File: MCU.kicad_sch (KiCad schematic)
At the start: 31 parts, among them J15 Display, J18 MEM2061-01-188-00-A_REVA, J19 TYPE-C 15PIN, Q1 PMBT6428,215, Q2 PMBT6428,215, SW5 Reset, SW6 Boot, U5 ESP32-WROOM-32E 4MB, U6 CP2102-GMR

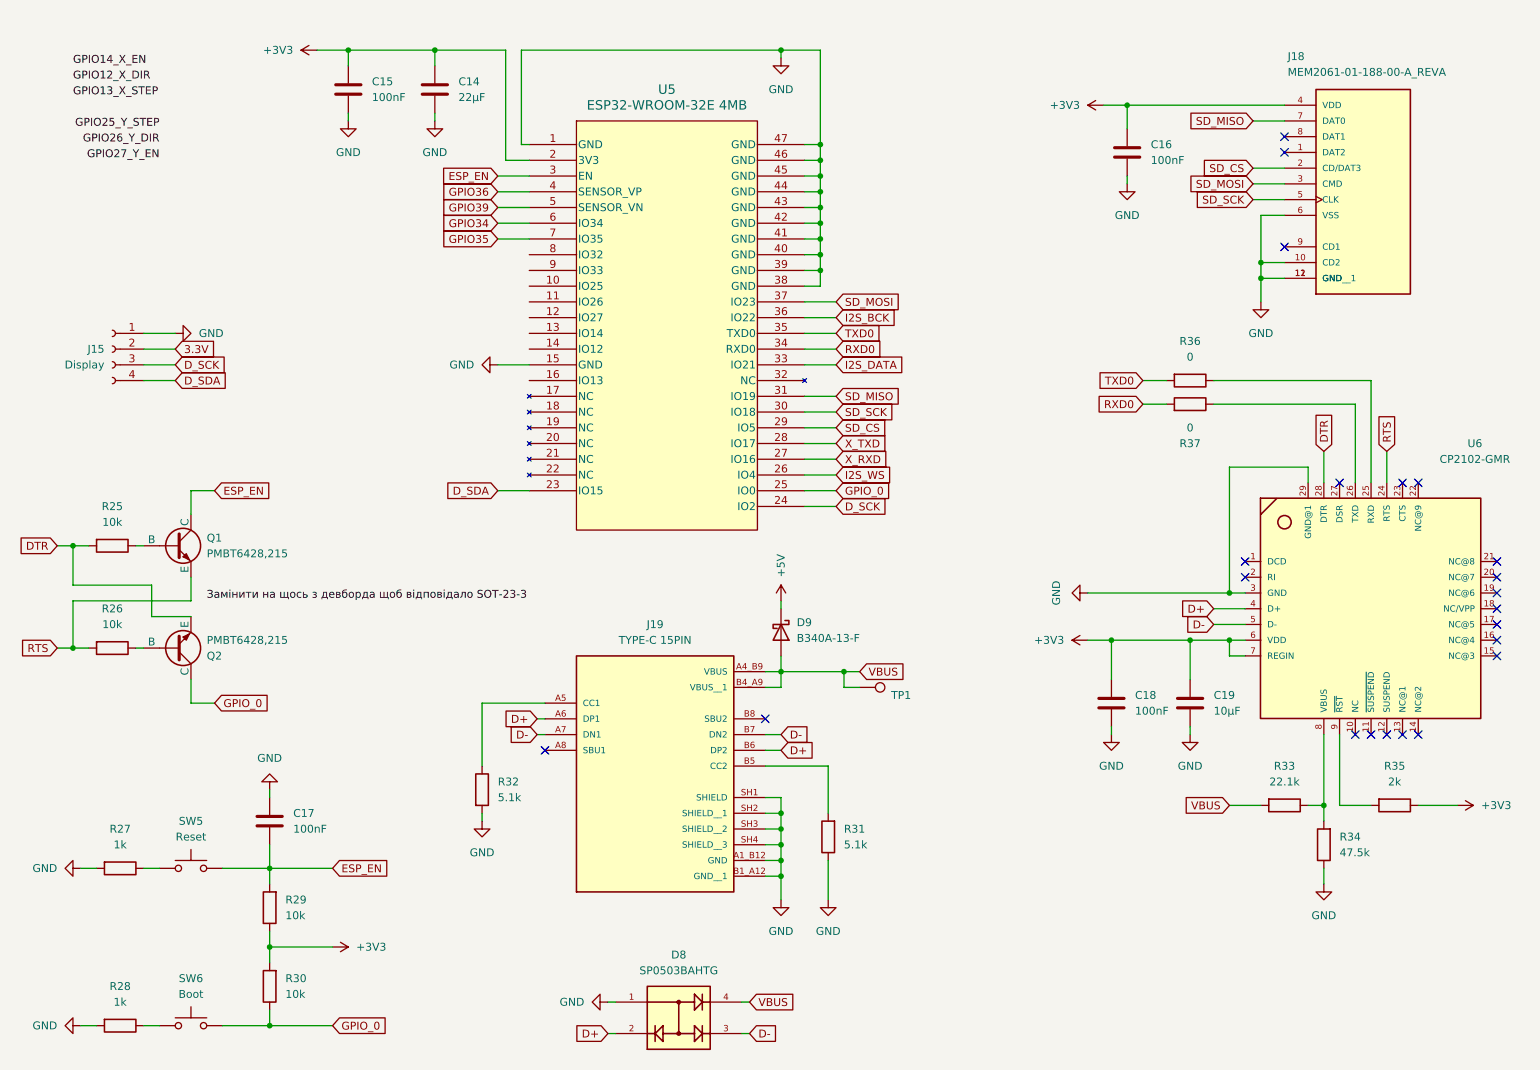
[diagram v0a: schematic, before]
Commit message: Finalization v2.0
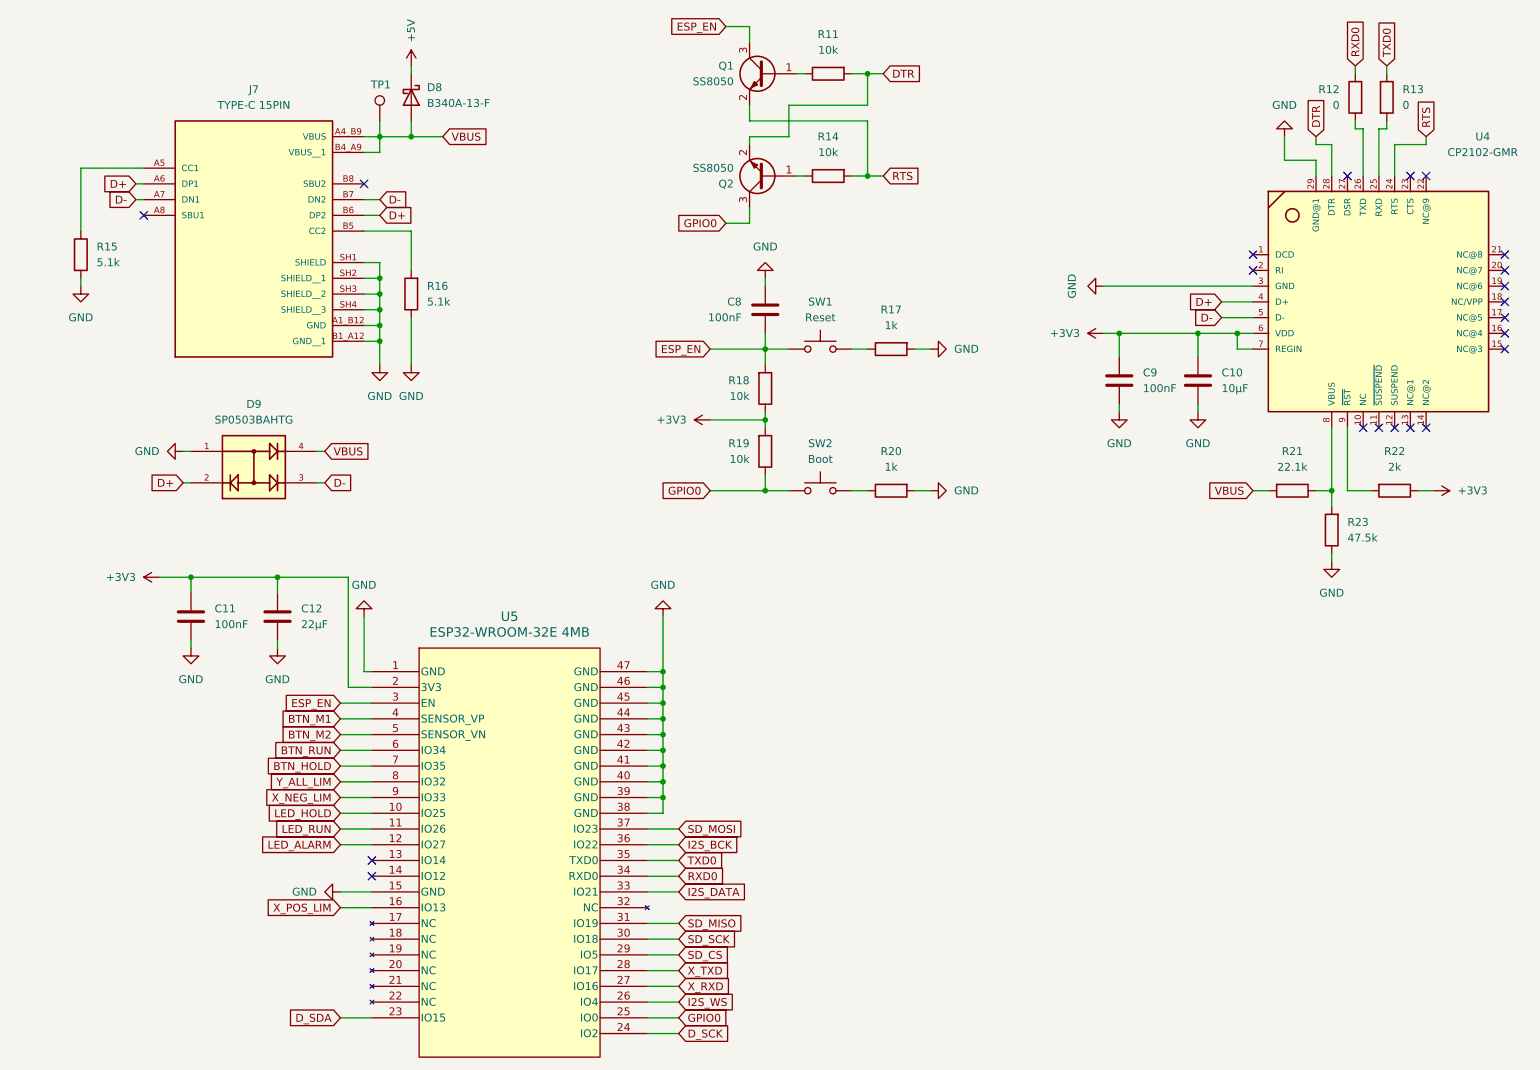
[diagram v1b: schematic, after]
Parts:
- removed C16: 100nF, Capacitor_SMD:C_0805_2012Metric_Pad1.18x1.45mm_HandSolder, symbol Device:C
- removed J15: Display, Connector_PinHeader_2.54mm:PinHeader_1x04_P2.54mm_Vertical, symbol Connector:Conn_01x04_Socket
- removed J18: MEM2061-01-188-00-A_REVA, MEM2061-01-188-00-A_REVA:GCT_MEM2061-01-188-00-A_REVA, symbol MEM2061_01_188_00_A:MEM2061-01-188-00-A_REVA
- removed Q1, Q2: PMBT6428,215, symbol Simulation_SPICE:NPN
- removed R37: 0, Resistor_SMD:R_0805_2012Metric_Pad1.20x1.40mm_HandSolder, symbol Device:R
- added Q1, Q2: SS8050, Package_TO_SOT_SMD:SOT-23, symbol Transistor_BJT:SS8050
- added R12: 0, Resistor_SMD:R_0805_2012Metric_Pad1.20x1.40mm_HandSolder, symbol Device:R
- J7: renamed from J19; footprint 10155435-00011LF:AMPHENOL_10155435-00011LF -> 10155435_00011LF:AMPHENOL_10155435-00011LF
- U4: renamed from U6; footprint INTERFACE-CP2102-GMR_QFN28_:QFN28G_0.5-5X5MM -> CP2102_GMR:QFN28G_0.5-5X5MM
- renumbered C19 to C10, C15 to C11, C14 to C12, C17 to C8, C18 to C9, D9 to D8, D8 to D9, R25 to R11, R36 to R13, R26 to R14, R32 to R15, R31 to R16, R27 to R17, R29 to R18, R30 to R19, R28 to R20, R33 to R21, R35 to R22, R34 to R23, SW5 to SW1, SW6 to SW2
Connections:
- net DTR: now also Q2.2 (E)
- net ESP_EN: now also Q1.3 (C)
- net RTS: now also Q1.2 (E)
- net RXD0: now also R12.1
- net TXD0: now also R13.1; no longer R13.2
- net at R11.1: now also Q1.1 (B)
- net at R14.1: now also Q2.1 (B)
- net at U4.25 (RXD): now also R13.2; no longer R13.1
- net at U4.26 (TXD): now also R12.2
- net LED_HOLD: now reaches U5.10 (IO25)
- net LED_RUN: now reaches U5.11 (IO26)
- net LED_ALARM: now reaches U5.12 (IO27)
- net X_POS_LIM: now reaches U5.16 (IO13)
- net Y_ALL_LIM: now reaches U5.8 (IO32)
- net X_NEG_LIM: now reaches U5.9 (IO33)
- net GPIO34 renamed BTN_RUN
- net GPIO35 renamed BTN_HOLD
- net GPIO36 renamed BTN_M1
- net GPIO39 renamed BTN_M2
- net GPIO_0 renamed GPIO0
- net GPIO0: now also Q2.3 (C)
- no-connect marks 22 -> 21
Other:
- moved on the sheet: C10, C11, C12, C8, C9, D8, D9, J7, R11, R13, R14, R15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
